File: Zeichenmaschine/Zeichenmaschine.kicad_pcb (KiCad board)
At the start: 2 copper layers, 39 parts, among them J1 interface_panel_0, J10 Conn_01x02_Male, J11 USB_C, J12 Conn_01x02_Male, J13 interface_panel_1, J14 Stepper_3_JUMPER, J15 Stepper_2, J2 Stepper_1, J3 Stepper_2, J4 Screw_Terminal_01x02, J5 Display, J6 Stepper_2_JUMPER, J7 Stepper_1_JUMPER, J8 dc_gear_motor, J9 SD_SPI, U1 TSR_1-2450, U2 L293D, U3 FT232RL

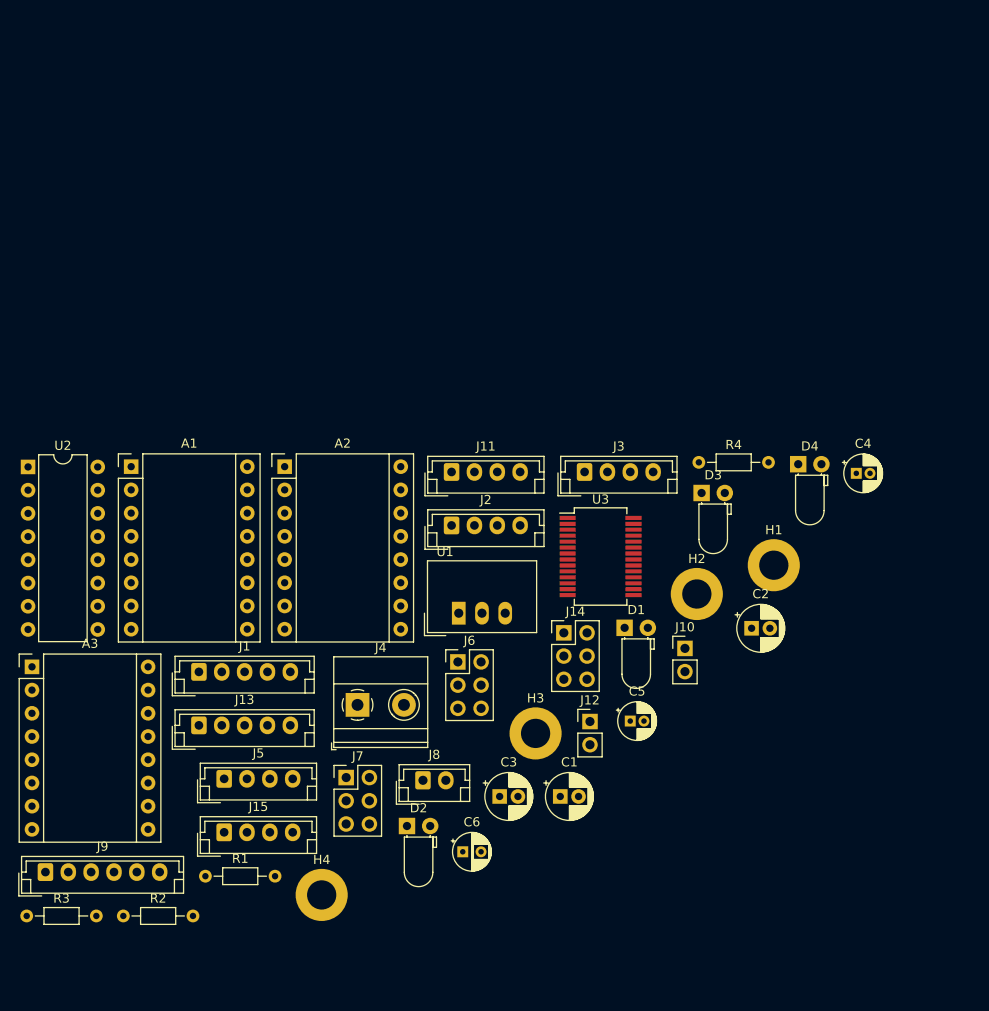
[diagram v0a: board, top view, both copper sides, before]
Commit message: asjhgdnsa
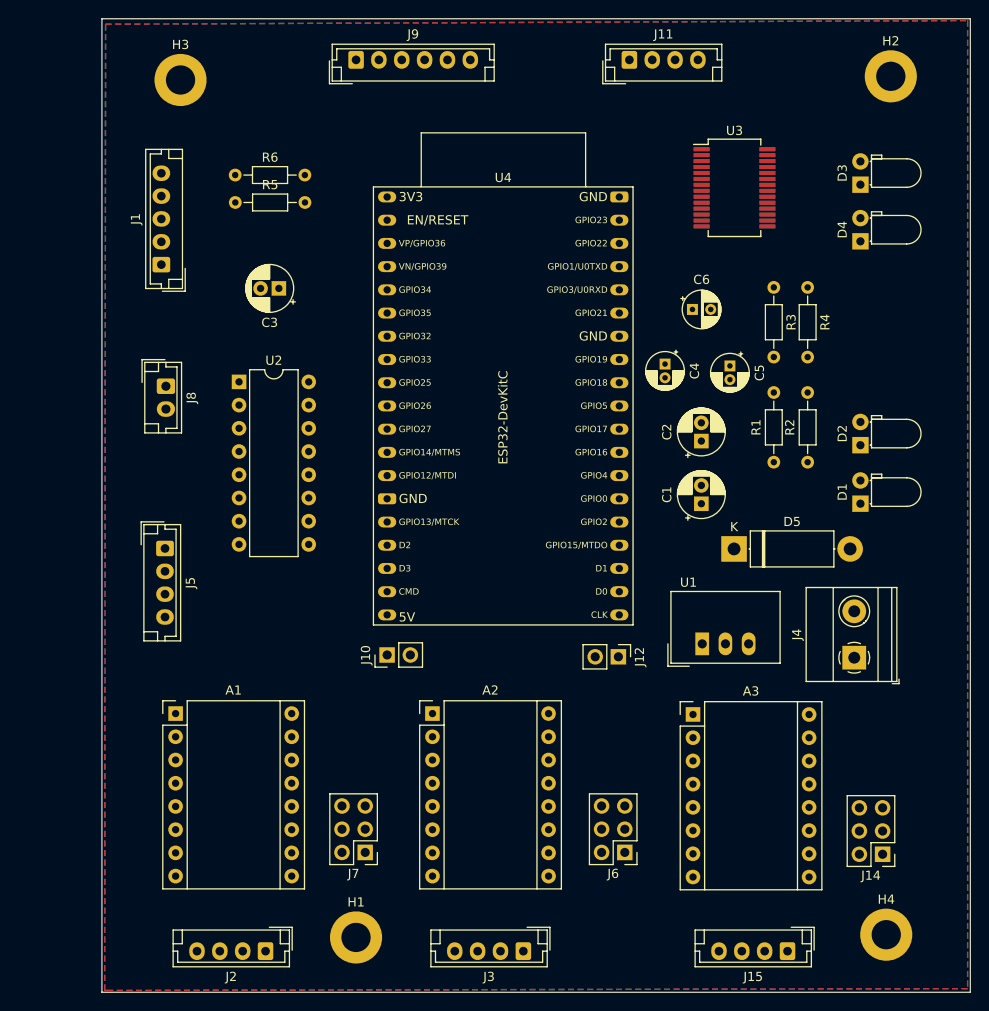
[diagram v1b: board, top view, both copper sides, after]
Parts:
- removed J13: interface_panel_1, Connector_JST:JST_EH_B5B-EH-A_1x05_P2.50mm_Vertical
- added D5: D_Schottky, Diode_THT:D_5W_P12.70mm_Horizontal, F.Cu at (180.2, 97.9)
- added R5: 1k, Resistor_THT:R_Axial_DIN0204_L3.6mm_D1.6mm_P7.62mm_Horizontal, F.Cu at (125.7, 60.0)
- added R6: 270, Resistor_THT:R_Axial_DIN0204_L3.6mm_D1.6mm_P7.62mm_Horizontal, F.Cu at (125.7, 57.0)
- added U4: ESP32-DevKitC, Espressif:ESP32-DevKitC, F.Cu at (142.3, 59.4)
- A3: value Stepper_2_A4988 -> Stepper_3_A4988
- J1: value interface_panel_0 -> interface
- J15: value Stepper_2 -> Stepper_3
- moved R3 106.8 mm to (184.6, 69.3), turned to -90 degrees
- moved J9 95.1 mm to (138.9, 44.4)
- moved R2 89.8 mm to (188.3, 88.4), turned to 90 degrees
- moved H3 81.4 mm to (119.7, 46.6)
- moved R1 76.9 mm to (184.6, 88.4), turned to 90 degrees
- moved A3 72.5 mm to (175.8, 116.0)
- moved D2 64.8 mm to (194.1, 86.5), turned to 90 degrees
- moved C6 64.4 mm to (175.7, 71.7)
- moved J15 63.0 mm to (186.1, 141.9), turned to 180 degrees
- moved H4 61.9 mm to (196.9, 140.1)
- moved H1 61.2 mm to (138.9, 140.4)
- moved C3 60.6 mm to (130.5, 69.4), turned to 180 degrees
- moved H2 60.5 mm to (197.4, 46.2)
- moved J4 54.6 mm to (193.4, 109.8), turned to 90 degrees
- moved J3 52.8 mm to (157.2, 141.9), turned to 180 degrees
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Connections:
- J1 pad 1: GND -> /interface_btn
- J1 pad 3: /UP -> Net-(J1-Pad3)
- J1 pad 4: /DN -> /interface_poti
- J1 pad 5: /PW -> +5V
- J15 pad 1: Net-(A3-Pad6) -> Net-(A3-Pad3)
- J15 pad 2: Net-(A3-Pad5) -> Net-(A3-Pad4)
- J15 pad 3: Net-(A3-Pad4) -> Net-(A3-Pad5)
- J15 pad 4: Net-(A3-Pad3) -> Net-(A3-Pad6)
- J2 pad 1: Net-(A1-Pad6) -> Net-(A1-Pad3)
- J2 pad 2: Net-(A1-Pad5) -> Net-(A1-Pad4)
- J2 pad 3: Net-(A1-Pad4) -> Net-(A1-Pad5)
- J2 pad 4: Net-(A1-Pad3) -> Net-(A1-Pad6)
- J3 pad 1: Net-(A2-Pad6) -> Net-(A2-Pad3)
- J3 pad 2: Net-(A2-Pad5) -> Net-(A2-Pad4)
- J3 pad 3: Net-(A2-Pad4) -> Net-(A2-Pad5)
- J3 pad 4: Net-(A2-Pad3) -> Net-(A2-Pad6)
- J4 pad 2: +12V -> Net-(J4-Pad2)
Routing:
- added copper zone on B.Cu, net GND
- added copper zone on F.Cu, net GND
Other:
- board outline added: 95 x 106.5 mm

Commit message: DrawMachine PCB V1
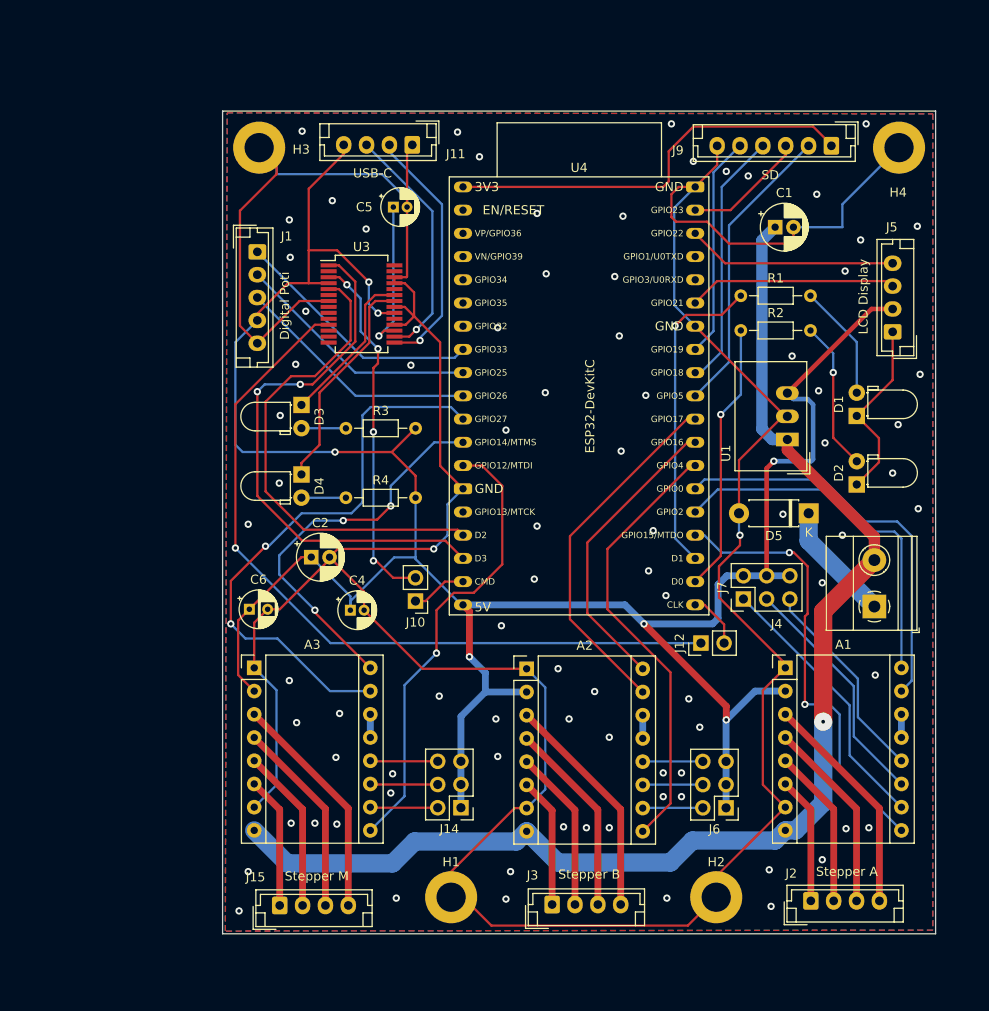
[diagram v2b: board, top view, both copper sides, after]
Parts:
- removed C3: C100_dc_gear_motor, Capacitor_THT:CP_Radial_D5.0mm_P2.00mm
- removed J8: dc_gear_motor, Connector_JST:JST_EH_B2B-EH-A_1x02_P2.50mm_Vertical
- removed R5: 1k, Resistor_THT:R_Axial_DIN0204_L3.6mm_D1.6mm_P7.62mm_Horizontal
- removed R6: 270, Resistor_THT:R_Axial_DIN0204_L3.6mm_D1.6mm_P7.62mm_Horizontal
- removed U2: L293D, Package_DIP:DIP-16_W7.62mm
- D5: footprint Diode_THT:D_5W_P12.70mm_Horizontal -> Diode_THT:D_DO-41_SOD81_P7.62mm_Horizontal
- moved H2 91.8 mm to (178.3, 136.0)
- moved H4 86.1 mm to (198.3, 54.0)
- moved J5 83.1 mm to (197.6, 74.2), turned to 90 degrees
- moved A1 66.9 mm to (185.9, 110.9)
- moved D4 66.3 mm to (132.9, 89.8), turned to -90 degrees
- moved D3 65.7 mm to (132.9, 82.2), turned to -90 degrees
- moved J2 59.9 mm to (188.7, 136.4), turned to 0 degrees
- moved C6 58.5 mm to (127.2, 104.5)
- moved J15 55.8 mm to (130.6, 136.9), turned to 0 degrees
- moved R4 55.5 mm to (137.8, 92.3), turned to 0 degrees
- moved J9 52.8 mm to (190.9, 53.8), turned to 180 degrees
- moved J7 49.8 mm to (181.3, 103.4), turned to 90 degrees
- moved R3 49.3 mm to (137.8, 84.7), turned to 0 degrees
- moved A3 48.3 mm to (127.8, 110.9)
- moved J14 46.4 mm to (150.4, 126.2)
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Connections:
- A1 pad 15: /Stepper_1_STEP -> /stepper_gear_motor_1A
- A1 pad 16: /Stepper_1_DIR -> /stepper_gear_motor_2A
- A1 pad 9: /enable_Stepper_1 -> /enable_stepper_gear_motor
- A3 pad 15: /dc_gear_motor_1A -> /Stepper_1_STEP
- A3 pad 16: /dc_gear_motor_2A -> /Stepper_1_DIR
- A3 pad 9: /enable_dc_gear_motor -> /enable_Stepper_1
- C4 pad 1: Net-(C4-Pad1) -> +5V
- C6 pad 1: Net-(C4-Pad1) -> +5V
- D5 pad 1: +12V -> Net-(D5-Pad1)
- D5 pad 2: Net-(J4-Pad2) -> GND
- J1 pad 1: /interface_btn -> /interface_CLK
- J1 pad 2: +5V -> /interface_DT
- J1 pad 3: Net-(J1-Pad3) -> /interface_SW
- J1 pad 4: /interface_poti -> +5V
- J1 pad 5: +5V -> GND
- J11 pad 4: Net-(C4-Pad1) -> +5V
- J15 pad 1: Net-(A3-Pad3) -> Net-(A3-Pad6)
- J15 pad 2: Net-(A3-Pad4) -> Net-(A3-Pad5)
- J15 pad 3: Net-(A3-Pad5) -> Net-(A3-Pad4)
- J15 pad 4: Net-(A3-Pad6) -> Net-(A3-Pad3)
- J2 pad 1: Net-(A1-Pad3) -> Net-(A1-Pad6)
- J2 pad 2: Net-(A1-Pad4) -> Net-(A1-Pad5)
- J2 pad 3: Net-(A1-Pad5) -> Net-(A1-Pad4)
- J2 pad 4: Net-(A1-Pad6) -> Net-(A1-Pad3)
- J3 pad 1: Net-(A2-Pad3) -> Net-(A2-Pad6)
- J3 pad 2: Net-(A2-Pad4) -> Net-(A2-Pad5)
- J3 pad 3: Net-(A2-Pad5) -> Net-(A2-Pad4)
- J3 pad 4: Net-(A2-Pad6) -> Net-(A2-Pad3)
- J4 pad 1: GND -> Net-(D5-Pad1)
- J4 pad 2: Net-(J4-Pad2) -> +12V
- J7 pad 1: +5V -> Net-(A1-Pad10)
- J7 pad 2: Net-(A1-Pad10) -> +5V
- J7 pad 3: +5V -> Net-(A1-Pad11)
- J7 pad 4: Net-(A1-Pad11) -> +5V
- J7 pad 5: +5V -> Net-(A1-Pad12)
- J7 pad 6: Net-(A1-Pad12) -> +5V
- R3 pad 2: Net-(C4-Pad1) -> +5V
- R4 pad 2: Net-(C4-Pad1) -> +5V
- U3 pad 20: Net-(C4-Pad1) -> +5V
- U4 pad 10: /interface_btn -> /interface_SW
- U4 pad 11: /enable_dc_gear_motor -> /Stepper_1_STEP
- U4 pad 12: /dc_gear_motor_1A -> /Stepper_1_DIR
- U4 pad 13: /dc_gear_motor_2A -> /enable_Stepper_1
- U4 pad 16: /L_R -> /RX
- U4 pad 17: /L_G -> /TX
- U4 pad 23: /enable_Stepper_1 -> /enable_stepper_gear_motor
- U4 pad 24: /Stepper_1_STEP -> /stepper_gear_motor_2A
- U4 pad 25: /Stepper_1_DIR -> /stepper_gear_motor_1A
- U4 pad 34: /RX -> unconnected-(U4-Pad34)
- U4 pad 35: /TX -> unconnected-(U4-Pad35)
- U4 pad 8: unconnected-(U4-Pad8) -> /interface_CLK
- U4 pad 9: /interface_poti -> /interface_DT
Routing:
- net GND: track 0.00 -> 404.6 mm, vias 0 -> 87
- net +5V: track 0.00 -> 276.3 mm, vias 0 -> 7
- net +12V: track 0.00 -> 141.2 mm, vias 0 -> 1
- net /CTS: track 0.00 -> 84.8 mm, vias 0 -> 1
- net /Stepper_1_STEP: track 0.00 -> 62.4 mm, vias 0 -> 2
- net /TX: track 0.00 -> 59.9 mm, vias 0 -> 2
- net /RX: track 0.00 -> 52.7 mm
- net /enable_Stepper_1: track 0.00 -> 50.2 mm, vias 0 -> 1
- net /enable_stepper_gear_motor: track 0.00 -> 48.7 mm, vias 0 -> 2
- net /enable_Stepper_2: track 0.00 -> 48.4 mm
- net +3V3: track 0.00 -> 45.9 mm
- net /stepper_gear_motor_1A: track 0.00 -> 44.1 mm
- net /Stepper_1_DIR: track 0.00 -> 42.9 mm, vias 0 -> 3
- net /stepper_gear_motor_2A: track 0.00 -> 39.9 mm
- net /RTS: track 0.00 -> 39.5 mm, vias 0 -> 4
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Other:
- board size 95 x 106.5 mm -> 78 x 90 mm
- board text added: "Digital Poti"
- board text added: "Drawmachine V1"
- board text added: "LCD Display"
- board text added: "SD"
- board text added: "Stepper A"
- board text added: "Stepper B"
- board text added: "Stepper M"
- board text added: "USB-C"
